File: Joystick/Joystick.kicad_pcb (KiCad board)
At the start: 2 copper layers, 70.1 x 70 mm, 13 parts, among them J1 Joystick, SW1 Plus, SW2 Minus, SW3 Down, SW4 Up, SW5 Right, SW6 Left, SW7 Center, U1 HDSP-A153, U2 AS1115-BSST

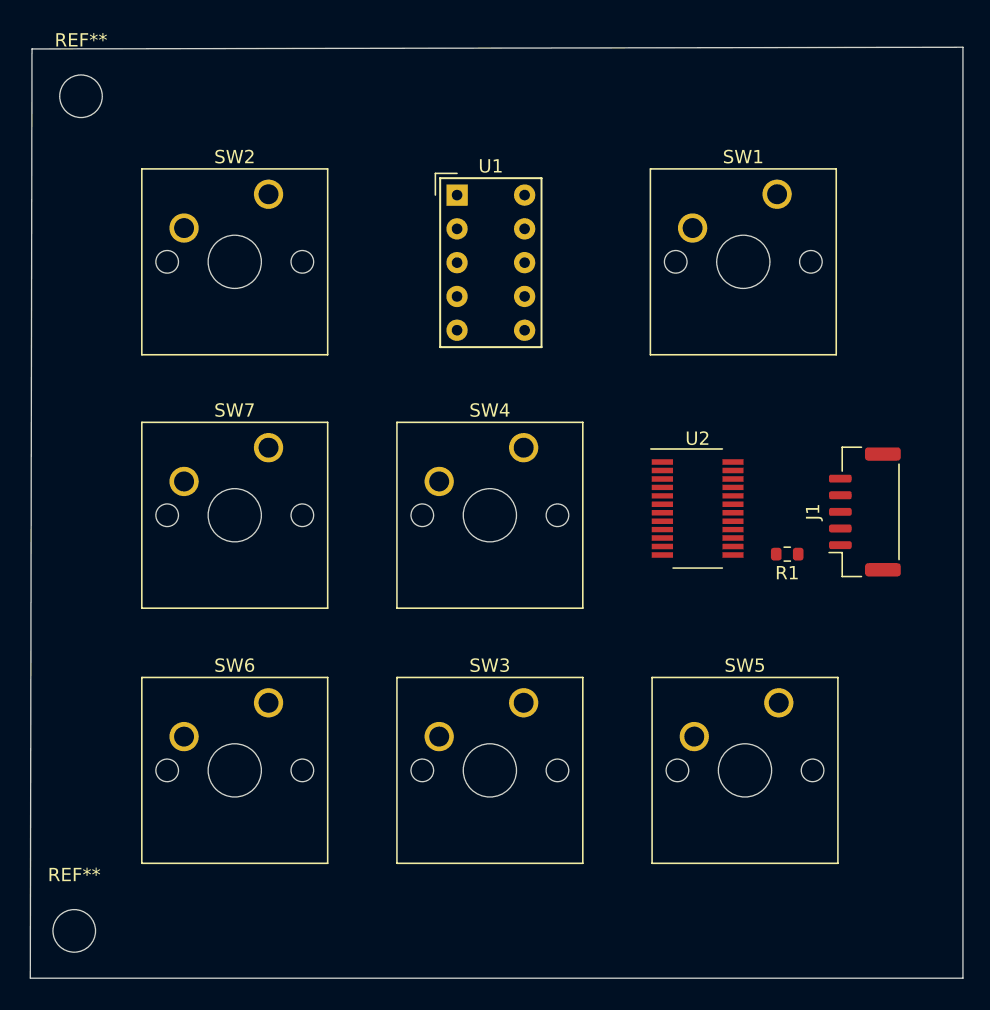
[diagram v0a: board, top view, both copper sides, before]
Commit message: keypad
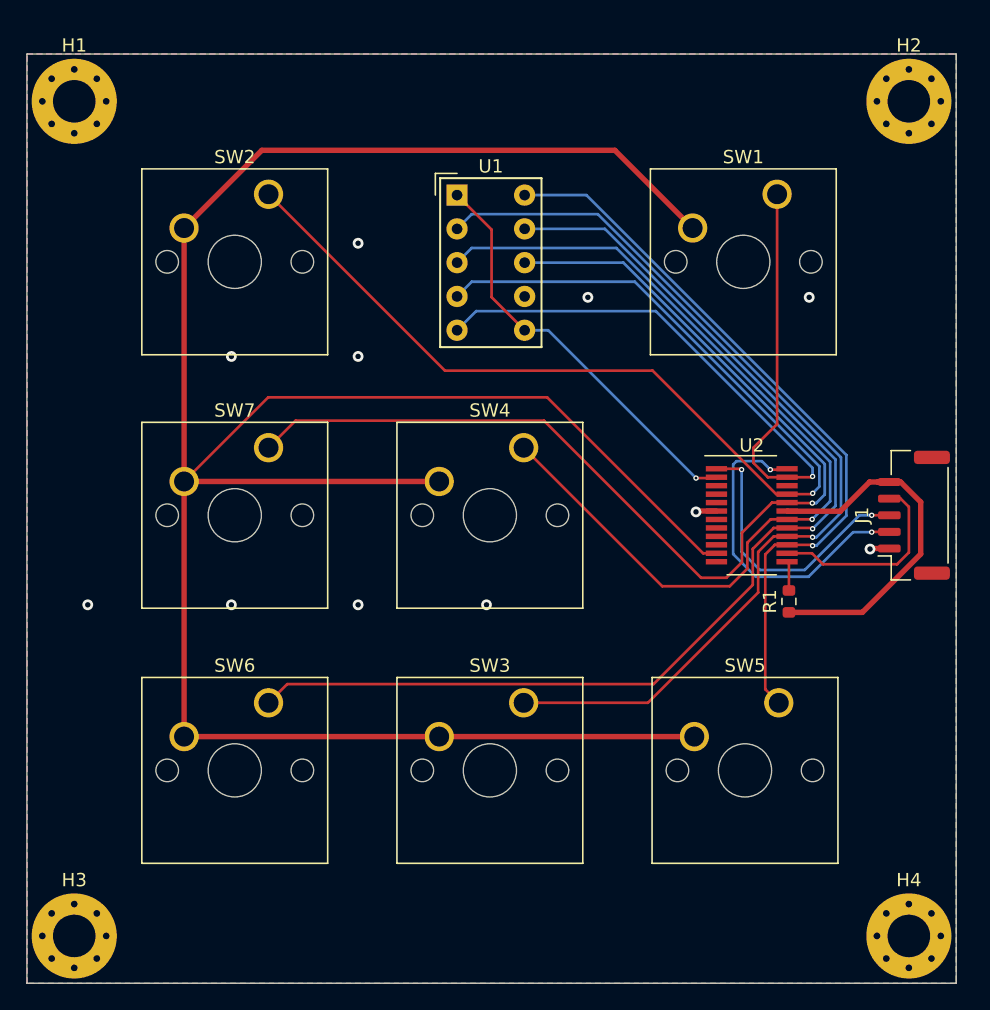
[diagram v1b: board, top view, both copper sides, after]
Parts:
- removed REF** (x2): MountingHole_3.2mm_M3, MountingHole:MountingHole_3.2mm_M3
- added G***: LOGO, Joystick:asian_tiger, F.Cu at (172.2, 102.0)
- added H1: *, MountingHole:MountingHole_3.2mm_M3_Pad_Via, F.Cu at (123.8, 66.4)
- added H2: *, MountingHole:MountingHole_3.2mm_M3_Pad_Via, F.Cu at (186.6, 66.4)
- added H3: *, MountingHole:MountingHole_3.2mm_M3_Pad_Via, F.Cu at (123.8, 129.2)
- added H4: *, MountingHole:MountingHole_3.2mm_M3_Pad_Via, F.Cu at (186.6, 129.2)
- moved U2 4.10 mm to (174.8, 97.5)
- moved J1 3.69 mm to (186.9, 97.5)
- moved R1 3.56 mm to (177.5, 104.0), turned to 90 degrees
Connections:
- SW2 pad 2: Net-(SW1-Pad1) -> Net-(SW1-Pad2)
- SW3 pad 1: Net-(SW1-Pad1) -> Net-(SW3-Pad1)
- SW3 pad 2: Net-(SW3-Pad2) -> Net-(SW1-Pad2)
- SW4 pad 2: Net-(SW1-Pad1) -> Net-(SW1-Pad2)
- SW5 pad 1: Net-(SW1-Pad1) -> Net-(SW5-Pad1)
- SW5 pad 2: Net-(SW5-Pad2) -> Net-(SW1-Pad2)
- SW6 pad 2: Net-(SW1-Pad1) -> Net-(SW1-Pad2)
- SW7 pad 1: Net-(SW1-Pad1) -> Net-(SW7-Pad1)
- SW7 pad 2: Net-(SW7-Pad2) -> Net-(SW1-Pad2)
- U1 pad 10: Net-(SW1-Pad2) -> Net-(SW5-Pad1)
- U1 pad 2: Net-(SW4-Pad1) -> Net-(SW3-Pad1)
- U1 pad 3: Net-(SW2-Pad1) -> Net-(SW4-Pad1)
- U1 pad 4: Net-(SW6-Pad1) -> Net-(SW2-Pad1)
- U1 pad 5: Net-(SW7-Pad2) -> Net-(SW1-Pad1)
- U1 pad 8: Net-(SW5-Pad2) -> Net-(SW7-Pad1)
- U1 pad 9: Net-(SW3-Pad2) -> Net-(SW6-Pad1)
- U2 pad 11: Net-(SW1-Pad1) -> Net-(SW1-Pad2)
- U2 pad 15: Net-(SW1-Pad2) -> Net-(SW5-Pad1)
- U2 pad 16: Net-(SW4-Pad1) -> Net-(SW3-Pad1)
- U2 pad 17: Net-(SW3-Pad2) -> Net-(SW6-Pad1)
- U2 pad 18: Net-(SW2-Pad1) -> Net-(SW4-Pad1)
- U2 pad 20: Net-(SW5-Pad2) -> Net-(SW7-Pad1)
- U2 pad 21: Net-(SW6-Pad1) -> Net-(SW2-Pad1)
- U2 pad 23: Net-(SW7-Pad2) -> Net-(SW1-Pad1)
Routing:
- net Net-(SW1-Pad2): track 0.00 -> 186.3 mm
- net Net-(SW2-Pad1): track 0.00 -> 85.9 mm, vias 0 -> 1
- net Net-(SW6-Pad1): track 0.00 -> 84.4 mm, vias 0 -> 1
- net Net-(SW7-Pad1): track 0.00 -> 82.7 mm, vias 0 -> 1
- net Net-(SW3-Pad1): track 0.00 -> 72.7 mm, vias 0 -> 1
- net Net-(SW4-Pad1): track 0.00 -> 69.3 mm, vias 0 -> 1
- net Net-(SW1-Pad1): track 0.00 -> 58.7 mm, vias 0 -> 1
- net Net-(SW5-Pad1): track 0.00 -> 55.8 mm, vias 0 -> 1
- net Net-(U1-Pad1): track 0.00 -> 31.3 mm, vias 0 -> 1
- net VCC: track 0.00 -> 28.1 mm
- net /IRQ: track 0.00 -> 25.0 mm, vias 0 -> 2
- net /SDA: track 0.00 -> 21.5 mm, vias 0 -> 2
- net /SCL: track 0.00 -> 15.0 mm
- net GND: track 0.00 -> 3.03 mm, vias 0 -> 11
- net Net-(R1-Pad2): track 0.00 -> 2.31 mm
- added copper zone on B.Cu, net GND
- added copper zone on F.Cu, net GND
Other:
- board size 70.1 x 70 mm -> 69.8 x 69.8 mm
- net class Default: clearance 0.2 -> 0.2032; trace_width 0.25 -> 0.2032; via_dia 0.8 -> 0.4064; via_drill 0.4 -> 0.2032
- net class Power added: clearance 0.2032, trace_width 0.4064, via_dia 0.8128, via_drill 0.4064
- rule trace_clearance: 0.2 -> 0.2032
- rule trace_min: 0.2 -> 0.2032
- rule via_min_drill: 0.3 -> 0.2032
- rule via_min_size: 0.4 -> 0.4064
- board text added: "Celestron Keypad v1.0 by Hyiger Designs"
